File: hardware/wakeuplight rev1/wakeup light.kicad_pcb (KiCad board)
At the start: 2 copper layers, 50 x 50 mm, 20 parts, among them J1 Serial_Header, J2 1/8_MH, J3 1/8_MH, J4 1/8_MH, J5 1/8_MH, J6 BARREL_JACK, J7 LED_Header, J8 Fog_Light, SW1 Rotary_Encoder, U1 Arduino_Pro_Mini, U2 Arduino_Nano, U3 LCD16x2, U4 CSD88539ND, U5 CSD88539ND

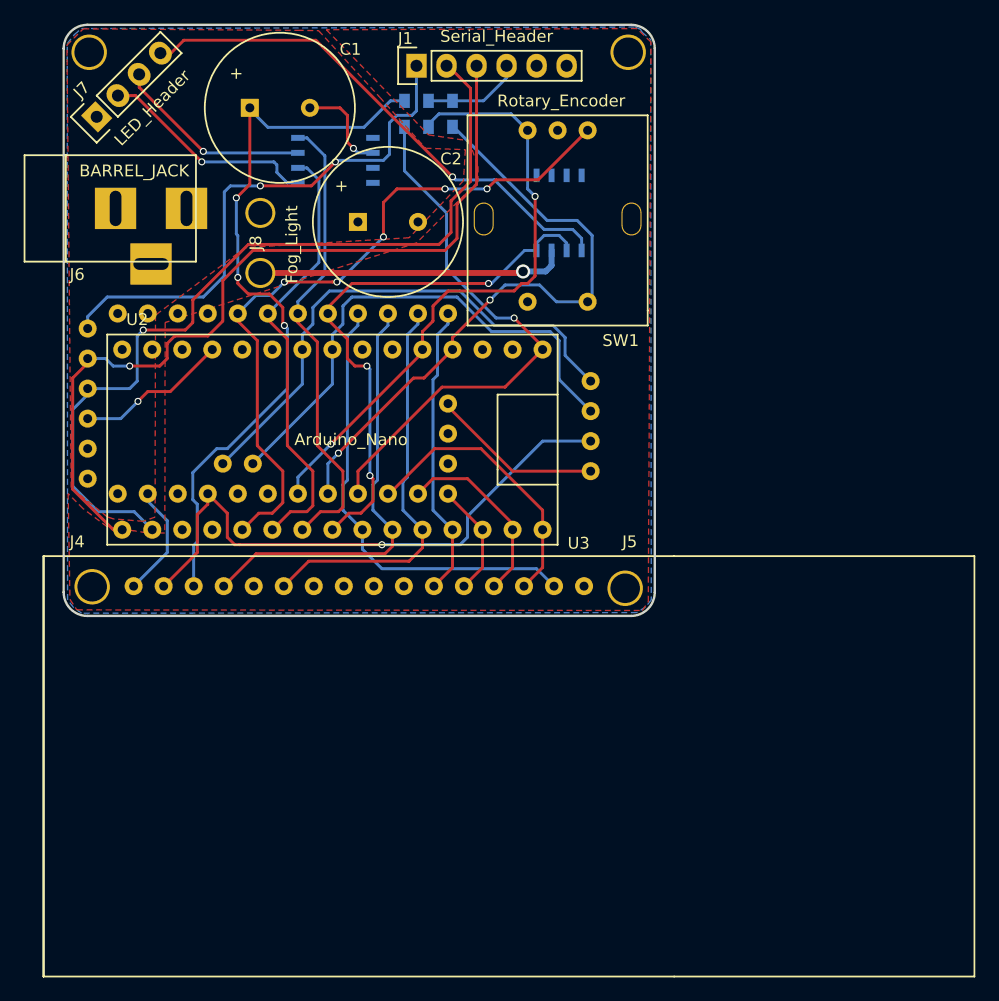
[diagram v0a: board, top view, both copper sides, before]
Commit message: Boards ordered!
gerbers generated and are on the way.
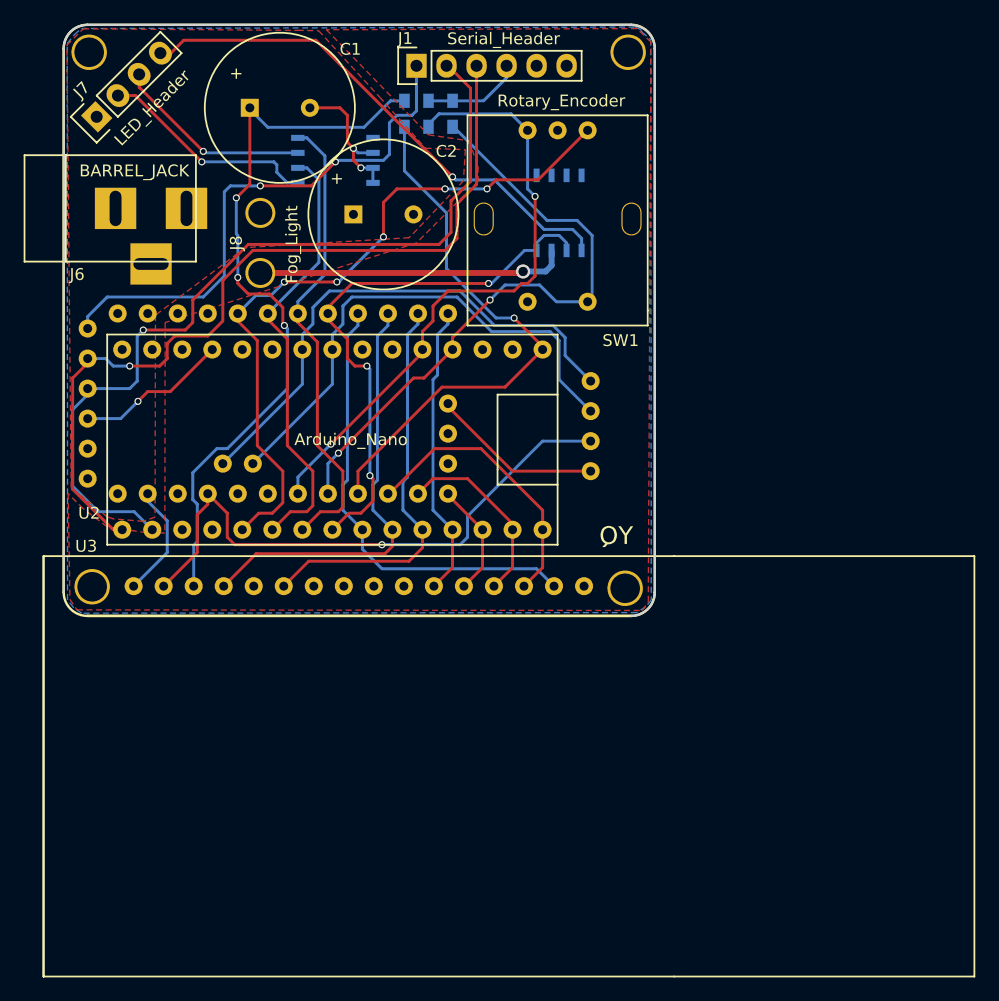
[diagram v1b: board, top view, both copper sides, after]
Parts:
- moved C2 0.74 mm to (81.4, 70.4)
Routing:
- net GND: track 32.5 -> 36.7 mm, vias 1 -> 2
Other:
- outline, holes or cut-outs redrawn
- board text added: "Wake-up Light Rev 1.0 Designed in ON, Canada"
- board text added: "YQ"
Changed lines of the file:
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@@
   (general
     (links 86)
-    (no_connects 2)
-    (area 56.796799 52.950799 106.996801 103.150801)
+    (no_connects 0)
+    (area 37.742819 44.958247 138.578001 134.0032)
     (thickness 1.6)
-    (drawings 9)
-    (tracks 378)
+    (drawings 19)
+    (tracks 383)
     (zones 0)
     (modules 20)
@@
   (layers
     (0 F.Cu signal)
-    (31 B.Cu signal hide)
+    (31 B.Cu signal)
     (32 B.Adhes user hide)
     (33 F.Adhes user hide)
@@
     (42 Eco1.User user hide)
     (43 Eco2.User user hide)
-    (44 Edge.Cuts user)
+    (44 Edge.Cuts user hide)
     (45 Margin user hide)
     (46 B.CrtYd user hide)
@@
     (pad_to_mask_clearance 0.2)
     (aux_axis_origin 0 0)
-    (visible_elements FFFFFF7F)
+    (visible_elements 7FFFFF7F)
     (pcbplotparams
-      (layerselection 0x00030_80000001)
-      (usegerberextensions false)
+      (layerselection 0x010fc_80000001)
+      (usegerberextensions true)
       (excludeedgelayer true)
       (linewidth 0.100000)
       (plotframeref false)
-      (viasonmask false)
+      (viasonmask true)
       (mode 1)
       (useauxorigin false)
@@
       (outputformat 1)
       (mirror false)
-      (drillshape 1)
+      (drillshape 0)
       (scaleselection 1)
-      (outputdirectory ""))
+      (outputdirectory gerbers/))
   )
   (net 0 "")
@@
     (add_net /FogLightReturn)
   )
+  (module "wakeuplight rev1:Cap_Fat_1000uF_25V" (layer F.Cu)
+    (at 81.407 70.358)
+    (fp_text reference C2 (at 7.874 -6.604) (layer F.SilkS)
+      (effects (font (size 1 1) (thickness 0.15)))
+    )
+    (fp_text value CP (at 3.81 12.319) (layer F.Fab) hide
+      (effects (font (size 1 1) (thickness 0.15)))
+    )
+    (fp_text user + (at -1.397 -4.318) (layer F.SilkS)
+      (effects (font (size 1 1) (thickness 0.15)))
+    )
+    (fp_circle (center 2.54 -1.27) (end -3.81 -1.27) (layer F.SilkS) (width 0.15))
+    (pad 1 thru_hole rect (at 0 -1.27) (size 1.524 1.524) (drill 0.762) (layers *.Cu *.Mask F.SilkS)
+      (net 3 +12V))
+    (pad 2 thru_hole circle (at 5.08 -1.27) (size 1.524 1.524) (drill 0.762) (layers *.Cu *.Mask F.SilkS)
+      (net 2 GND))
+  )
   (module Pin_Headers:Pin_Header_Straight_1x04 (layer F.Cu)
     (at 59.69 60.833 135)
@@
   (module "wakeuplight rev1:Arduino_Nano" (layer F.Cu)
     (at 80.899 86.868)
-    (fp_text reference U2 (at -17.78 -8.89) (layer F.SilkS)
+    (fp_text reference U2 (at -21.844 7.493) (layer F.SilkS)
       (effects (font (size 1 1) (thickness 0.15)))
     )
@@
       (net 2 GND))
   )
-  (module "wakeuplight rev1:Cap_Fat_1000uF_25V" (layer F.Cu)
-    (at 81.788 70.993)
-    (fp_text reference C2 (at 7.874 -6.604) (layer F.SilkS)
-      (effects (font (size 1 1) (thickness 0.15)))
-    )
-    (fp_text value CP (at 3.81 12.319) (layer F.Fab) hide
-      (effects (font (size 1 1) (thickness 0.15)))
-    )
-    (fp_text user + (at -1.397 -4.318) (layer F.SilkS)
-      (effects (font (size 1 1) (thickness 0.15)))
-    )
-    (fp_circle (center 2.54 -1.27) (end -3.81 -1.27) (layer F.SilkS) (width 0.15))
-    (pad 1 thru_hole rect (at 0 -1.27) (size 1.524 1.524) (drill 0.762) (layers *.Cu *.Mask F.SilkS)
-      (net 3 +12V))
-    (pad 2 thru_hole circle (at 5.08 -1.27) (size 1.524 1.524) (drill 0.762) (layers *.Cu *.Mask F.SilkS)
-      (net 2 GND))
-  )
   (module Pin_Headers:Pin_Header_Straight_1x06 (layer F.Cu)
     (at 86.741 56.515 90)
@@
       (effects (font (size 1 1) (thickness 0.15)))
     )
-    (fp_text value Serial_Header (at 2.4892 6.7818 180) (layer F.SilkS)
+    (fp_text value Serial_Header (at 2.286 7.366 180) (layer F.SilkS)
       (effects (font (size 1 1) (thickness 0.15)))
     )
@@
     (tags "resistor 0603")
     (attr smd)
-    (fp_text reference R1 (at 0 1.9 270) (layer B.SilkS)
+    (fp_text reference R1 (at 3.175 0 270) (layer B.SilkS)
       (effects (font (size 1 1) (thickness 0.15)) (justify mirror))
     )
@@
     (tags "resistor 0603")
     (attr smd)
-    (fp_text reference R2 (at 0 1.9 270) (layer B.SilkS)
+    (fp_text reference R2 (at 3.175 0 270) (layer B.SilkS)
       (effects (font (size 1 1) (thickness 0.15)) (justify mirror))
     )
@@
     (tags "resistor 0603")
     (attr smd)
-    (fp_text reference R3 (at 0 1.9 270) (layer B.SilkS)
+    (fp_text reference R3 (at 3.175 0 270) (layer B.SilkS)
       (effects (font (size 1 1) (thickness 0.15)) (justify mirror))
     )
@@
   (module "wakeuplight rev1:LCD_16x2" (layer F.Cu)
     (at 62.8142 133.5532)
-    (fp_text reference U3 (at 37.6428 -36.6522) (layer F.SilkS)
+    (fp_text reference U3 (at -4.0132 -36.3982) (layer F.SilkS)
       (effects (font (size 1 1) (thickness 0.15)))
     )
@@
     (tags "CMS SOJ")
     (attr smd)
-    (fp_text reference U4 (at 3.3274 0.2032 270) (layer B.SilkS)
+    (fp_text reference U4 (at 3.937 0.127 270) (layer B.SilkS)
       (effects (font (size 1 1) (thickness 0.15)) (justify mirror))
     )
@@
     (tags "CMS SOJ")
     (attr smd)
-    (fp_text reference U5 (at 3.3528 0.254 180) (layer B.SilkS)
+    (fp_text reference U5 (at 3.683 0.254 180) (layer B.SilkS)
       (effects (font (size 1 1) (thickness 0.15)) (justify mirror))
     )
@@
   (module "wakeuplight rev1:2.5mm_MH" (layer F.Cu)
     (at 59.309 100.584)
-    (fp_text reference J4 (at -1.27 -3.81) (layer F.SilkS)
+    (fp_text reference J4 (at -5.969 -2.159) (layer F.SilkS) hide
       (effects (font (size 1 1) (thickness 0.15)))
     )
@@
   (module "wakeuplight rev1:2.5mm_MH" (layer F.Cu)
     (at 104.394 100.711)
-    (fp_text reference J5 (at 0.381 -3.937) (layer F.SilkS)
+    (fp_text reference J5 (at 6.731 -5.588) (layer F.SilkS) hide
       (effects (font (size 1 1) (thickness 0.15)))
     )
@@
   (module "wakeuplight rev1:Fog_Light" (layer F.Cu)
     (at 73.533 68.961 270)
-    (fp_text reference J8 (at 2.54 0.381 270) (layer F.SilkS)
+    (fp_text reference J8 (at 2.54 2.032 270) (layer F.SilkS)
       (effects (font (size 1 1) (thickness 0.15)))
     )
@@
       (net 48 /FogLightReturn))
   )
+  (gr_arc (start 104.8968 55.0508) (end 104.8968 53.0508) (angle 90) (layer F.SilkS) (width 0.2))
   (gr_line (start 106.8968 55.0508) (end 106.8968 101.0508) (angle 90) (layer Edge.Cuts) (width 0.2))
+  (gr_arc (start 104.8968 101.0508) (end 106.8968 101.0508) (angle 90) (layer F.SilkS) (width 0.2))
+  (gr_line (start 104.8968 103.0508) (end 58.8968 103.0508) (angle 90) (layer F.SilkS) (width 0.2))
+  (gr_line (start 56.8968 101.0508) (end 56.8968 55.0508) (angle 90) (layer F.SilkS) (width 0.2))
+  (gr_arc (start 58.8968 55.0508) (end 56.8968 55.0508) (angle 90) (layer Edge.Cuts) (width 0.2))
+  (gr_line (start 58.8968 53.0508) (end 104.8968 53.0508) (angle 90) (layer F.SilkS) (width 0.2))
+  (gr_text YQ (at 103.632 96.266) (layer B.SilkS)
+    (effects (font (size 1.5 1.5) (thickness 0.3)))
+  )
+  (gr_text YQ (at 103.632 96.266) (layer F.SilkS)
+    (effects (font (size 1.5 1.5) (thickness 0.3)) (justify mirror))
+  )
+  (gr_text "Wake-up Light\nRev 1.0\nDesigned in ON, Canada" (at 76.327 56.007) (layer B.SilkS)
+    (effects (font (size 0.6 0.6) (thickness 0.15)) (justify mirror))
+  )
+  (gr_line (start 106.8968 55.0508) (end 106.8968 101.0508) (angle 90) (layer F.SilkS) (width 0.2))
   (gr_line (start 58.8968 53.0508) (end 104.8968 53.0508) (angle 90) (layer Edge.Cuts) (width 0.2))
   (gr_line (start 56.8968 101.0508) (end 56.8968 55.0508) (angle 90) (layer Edge.Cuts) (width 0.2))
-  (gr_line (start 104.8968 103.0508) (end 58.8968 103.0508) (angle 90) (layer Edge.Cuts) (width 0.2))
+  (gr_line (start 104.8968 103.0508) (end 58.8968 103.0508) (angle 90) (layer F.SilkS) (width 0.2))
   (gr_arc (start 104.8968 55.0508) (end 104.8968 53.0508) (angle 90) (layer Edge.Cuts) (width 0.2))
-  (gr_arc (start 58.8968 55.0508) (end 56.8968 55.0508) (angle 90) (layer Edge.Cuts) (width 0.2))
-  (gr_arc (start 58.8968 101.0508) (end 58.8968 103.0508) (angle 90) (layer Edge.Cuts) (width 0.2))
+  (gr_arc (start 58.8968 55.0508) (end 56.8968 55.0508) (angle 90) (layer F.SilkS) (width 0.2))
+  (gr_arc (start 58.8968 101.0508) (end 58.8968 103.0508) (angle 90) (layer F.SilkS) (width 0.2))
   (gr_arc (start 104.8968 101.0508) (end 106.8968 101.0508) (angle 90) (layer Edge.Cuts) (width 0.2))
   (gr_line (start 106.06532 103.00716) (end 106.06532 103.01224) (angle 90) (layer F.Fab) (width 0.2))
@@
   (segment (start 82.296 61.722) (end 84.539 59.479) (width 0.25) (layer B.Cu) (net 1))
   (segment (start 84.539 59.479) (end 85.725 59.479) (width 0.25) (layer B.Cu) (net 1))
+  (segment (start 83.058 65.151) (end 83.058 66.421) (width 0.25) (layer B.Cu) (net 2))
+  (segment (start 83.058 65.151) (end 82.042 65.151) (width 0.25) (layer B.Cu) (net 2))
+  (segment (start 81.407 64.516) (end 81.407 63.5) (width 0.25) (layer F.Cu) (net 2))
+  (segment (start 82.042 65.151) (end 81.407 64.516) (width 0.25) (layer F.Cu) (net 2))
+  (via (at 82.042 65.151) (size 0.6) (drill 0.4) (layers F.Cu B.Cu) (net 2))
+  (segment (start 89.408 85.09) (end 89.408 85.344) (width 0.25) (layer F.Cu) (net 2))
+  (segment (start 89.408 85.344) (end 94.869 90.805) (width 0.25) (layer F.Cu) (net 2))
+  (segment (start 94.869 90.805) (end 101.473 90.805) (width 0.25) (layer F.Cu) (net 2))
   (segment (start 64.008 92.71) (end 64.008 93.345) (width 0.25) (layer B.Cu) (net 2))
   (segment (start 64.008 93.345) (end 65.659 94.996) (width 0.25) (layer B.Cu) (net 2))
   (segment (start 65.659 94.996) (end 65.659 97.6884) (width 0.25) (layer B.Cu) (net 2))
   (segment (start 65.659 97.6884) (end 62.8142 100.5332) (width 0.25) (layer B.Cu) (net 2))
-  (segment (start 89.408 85.09) (end 89.408 85.344) (width 0.25) (layer F.Cu) (net 2))
-  (segment (start 89.408 85.344) (end 94.869 90.805) (width 0.25) (layer F.Cu) (net 2))
-  (segment (start 94.869 90.805) (end 101.473 90.805) (width 0.25) (layer F.Cu) (net 2))
   (segment (start 77.724 60.071) (end 80.264 60.071) (width 0.25) (layer F.Cu) (net 2))
   (segment (start 81.788 63.881) (end 83.058 63.881) (width 0.25) (layer B.Cu) (net 2))
